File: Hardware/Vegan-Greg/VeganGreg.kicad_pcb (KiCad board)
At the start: 4 copper layers, 136 parts, among them J1 RBUS, J2 USB_C_Receptacle_USB2.0, J3 ServoCH0, J4 Conn_01x06_Socket, J5 GPIO Breakout, Q1 SSM3K15AMFV,L3F, U1 ESP32-S3, U2 SN65HVD230, U3 LM66200DRLR, U4 MAX77827AEFD+T, U5 SC4215ASTRT, U6 SIC438AED-T1, U7 LT1762, U8 TPS61089, Y1 R940000171

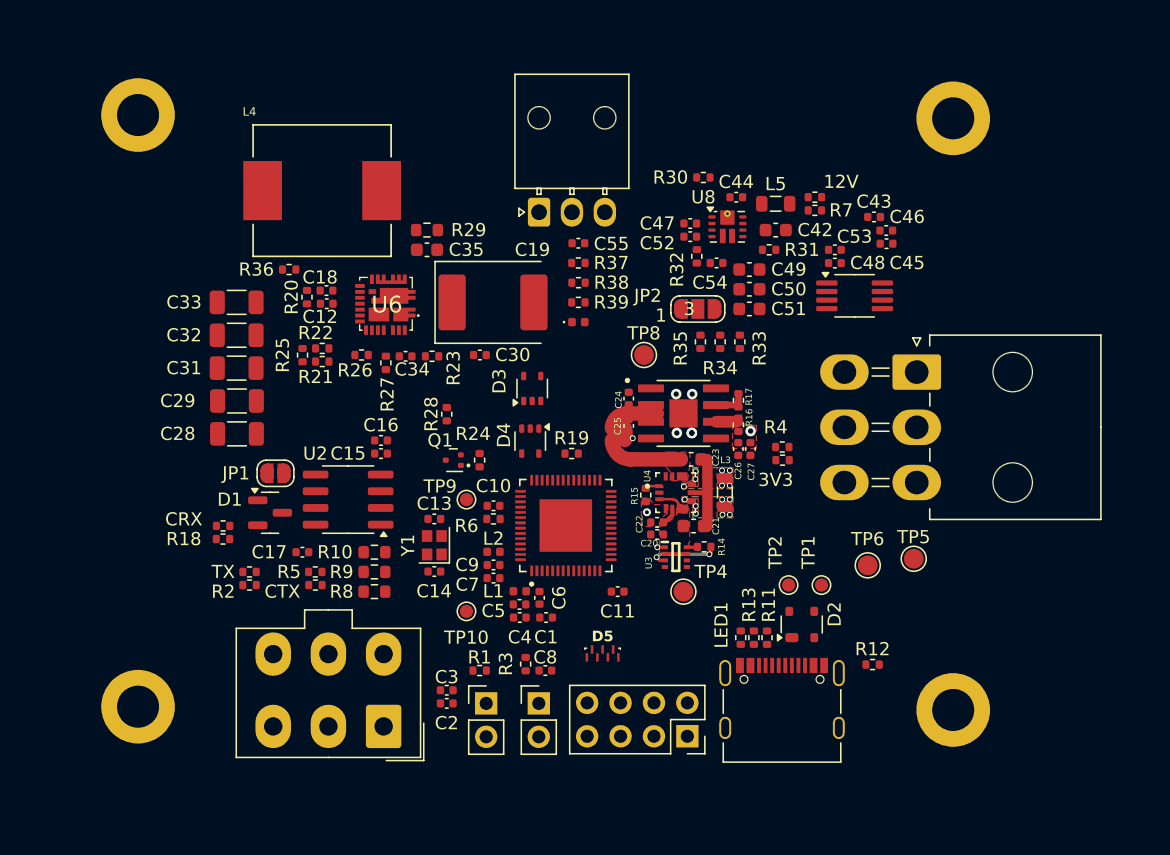
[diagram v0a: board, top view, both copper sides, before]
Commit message: Full PCB design
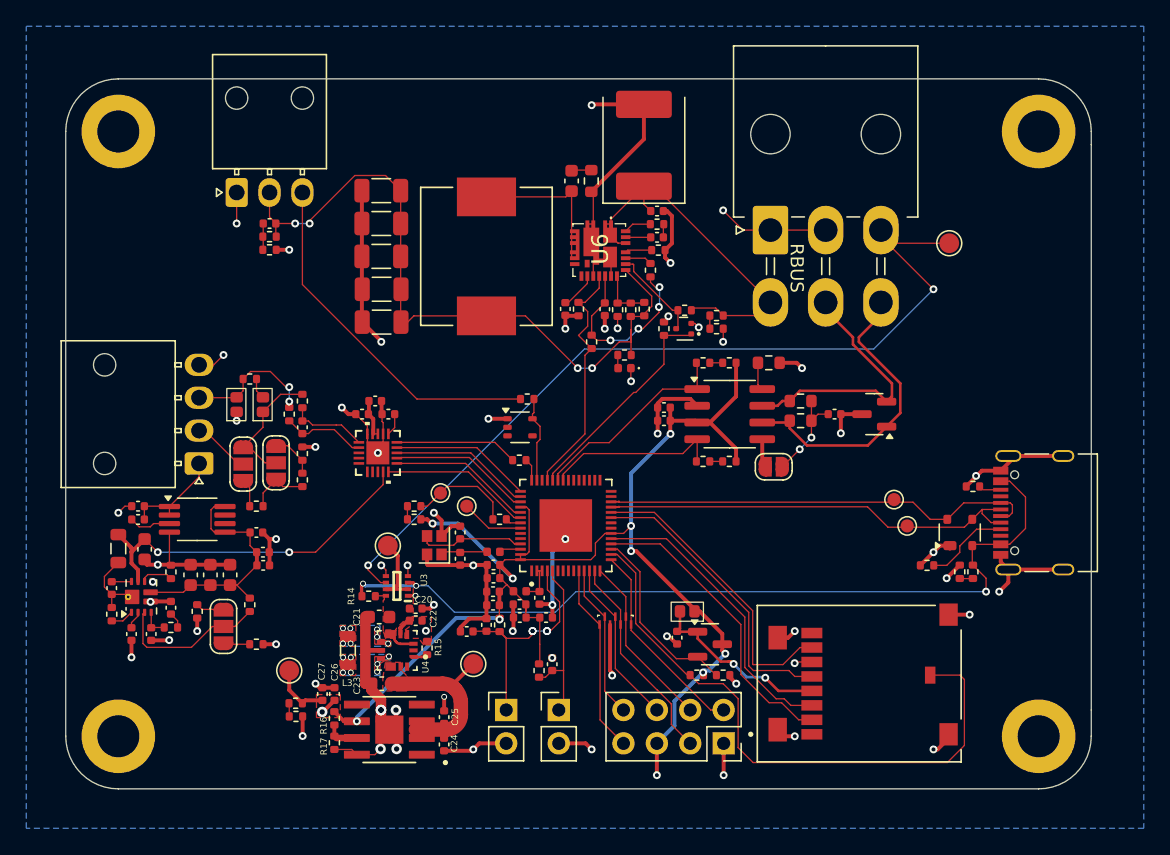
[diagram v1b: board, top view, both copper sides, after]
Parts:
- removed D3: ~, Package_TO_SOT_SMD:SOT-353_SC-70-5
- added C56: 10nF, Capacitor_SMD:C_0402_1005Metric, F.Cu at (134.9, 103.1)
- added C58: 220nF, Capacitor_SMD:C_0402_1005Metric, F.Cu at (141.5, 102.1)
- added C59: 1nF, Capacitor_SMD:C_0402_1005Metric, F.Cu at (140.5, 101.1)
- added C60: 1nF, Capacitor_SMD:C_0402_1005Metric, F.Cu at (139.5, 102.1)
- added C61: 0.1uF, Capacitor_SMD:C_0402_1005Metric, F.Cu at (163.4, 119.1)
- added J7: ST1W008S4TR2000, iclr:JAE_ST1W008S4TR2000, F.Cu at (177.4, 122.6)
- added JP13: SolderJumper_2_Open, iclr:SmallerSolderJP, F.Cu at (163.9, 117.1)
- added JP4: SolderJumper_3_Open, Jumper:SolderJumper-3_P1.3mm_Open_RoundedPad1.0x1.5mm_NumberLabels, F.Cu at (130.4, 105.9)
- added JP5: SolderJumper_3_Open, Jumper:SolderJumper-3_P1.3mm_Open_RoundedPad1.0x1.5mm_NumberLabels, F.Cu at (132.9, 105.8)
- added JP6: SolderJumper_2_Open, iclr:SmallerSolderJP, F.Cu at (131.9, 101.1)
- added JP7: SolderJumper_2_Open, iclr:SmallerSolderJP, F.Cu at (129.9, 101.1)
- added Q2: PMOS, Package_TO_SOT_SMD:SOT-23, F.Cu at (165.9, 119.6)
- added R46: 75k, Resistor_SMD:R_0402_1005Metric, F.Cu at (131.4, 109.1)
- added R47: 14k, Resistor_SMD:R_0402_1005Metric, F.Cu at (134.9, 107.1)
- added R48: 10k, Resistor_SMD:R_0402_1005Metric, F.Cu at (134.9, 105.1)
- added R49: 1k, Resistor_SMD:R_0402_1005Metric, F.Cu at (134.9, 101.1)
- added R50: 49.9, Resistor_SMD:R_0402_1005Metric, F.Cu at (130.9, 99.4)
- added R51: 1k, Resistor_SMD:R_0402_1005Metric, F.Cu at (133.9, 102.1)
- added R52: 54.9, Resistor_SMD:R_0402_1005Metric, F.Cu at (151.4, 105.6)
- added R59: 1k, Resistor_SMD:R_0402_1005Metric, F.Cu at (166.9, 121.9)
- added R60: 10k, Resistor_SMD:R_0402_1005Metric, F.Cu at (164.9, 121.9)
- added U9: ADS131M02IRUKR, footprints:WQFN20_ADS131_TEX, F.Cu at (140.7, 105.0)
- J1: footprint Connector_Molex:Molex_Mini-Fit_Jr_5566-06A_2x03_P4.20mm_Vertical -> iclr:Molex_Mini-Fit_Jr_5569-06A2_2x03_P4.20mm_Horizontal
- J4: value Conn_01x06_Socket -> 1053131104; footprint iclr:Molex_Mini-Fit_Jr_5569-06A2_2x03_P4.20mm_Horizontal -> Connector_Molex:Molex_Nano-Fit_105313-xx04_1x04_P2.50mm_Horizontal
- moved C48 56.5 mm to (122.4, 110.1)
- moved C53 56.5 mm to (122.4, 109.1)
- moved L5 56.5 mm to (120.9, 112.3), turned to -90 degrees
- moved C44 56.0 mm to (120.4, 115.3), turned to 90 degrees
- moved R30 55.9 mm to (120.4, 117.3), turned to -90 degrees
- moved J4 55.0 mm to (127.1, 105.8), turned to 180 degrees
- moved C42 53.8 mm to (122.9, 112.4), turned to -90 degrees
- moved C45 53.3 mm to (131.9, 113.6)
- moved C46 53.3 mm to (131.9, 112.6)
- moved U7 52.8 mm to (126.9, 110.1)
- moved C43 52.8 mm to (131.4, 111.1)
- moved C47 52.7 mm to (121.9, 118.8), turned to -90 degrees
- moved U8 52.7 mm to (122.7, 116.0), turned to 90 degrees
- moved R31 51.7 mm to (124.9, 114.1), turned to 90 degrees
- moved C52 50.9 mm to (123.4, 118.8), turned to -90 degrees
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- renumbered 12V to 12VLED1, 3V3 to 3V3LED1, CRX to CRXLED1, CTX to CTXLED1, TX to TXLED1, LED1 to USBLED1
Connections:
- C19 pad 1: +16.8V -> DeployV
- C30 pad 1: +16.8V -> DeployV
- C43 pad 1: Net-(U7-IN) -> 5_or_12
- C45 pad 1: /gregPart/LDO5.5V_IN -> 5_or_12
- C46 pad 1: /gregPart/LDO5.5V_IN -> 5_or_12
- C48 pad 1: Net-(U7-ADJ) -> LDO_out
- C49 pad 1: /gregPart/VOut - 5 or 12V -> 5_or_12
- C50 pad 1: /gregPart/VOut - 5 or 12V -> 5_or_12
- C51 pad 1: /gregPart/VOut - 5 or 12V -> 5_or_12
- C53 pad 1: Net-(U7-ADJ) -> LDO_out
- J1 pad 4: +25.2V -> DeployV
- J4 pad 1: GND -> LDO_out
- J4 pad 2: GND -> Net-(JP4-C)
- J4 pad 3: RBUS_uC_V -> Net-(JP7-B)
- J4 pad 4: +12V -> GND
- R28 pad 2: +16.8V -> DeployV
- R34 pad 1: /gregPart/VOut - 5 or 12V -> 5_or_12
- R7 pad 1: 25.2V -> DeployV
- U1 pad 16: unconnected-(U1-GPIO11/ADC2_CH0-Pad16) -> /SD_DET
- U1 pad 17: unconnected-(U1-GPIO12/ADC2_CH1-Pad17) -> /SD_EN
- U1 pad 18: unconnected-(U1-GPIO13/ADC2_CH2-Pad18) -> /SD_CS
- U1 pad 19: unconnected-(U1-GPIO14/ADC2_CH3-Pad19) -> /VSPI_MOSI
- U1 pad 23: unconnected-(U1-GPIO17/ADC2_CH6/DAC_2-Pad23) -> /VSPI_SCLK
- U1 pad 24: unconnected-(U1-GPIO18/ADC2_CH7/DAC_1-Pad24) -> /VSPI_MISO
- U1 pad 36: unconnected-(U1-SPICLK_N/GPIO48-Pad36) -> /CAN_RX
- U1 pad 37: /BuckPGOOD -> /CAN_TX
- U1 pad 38: /CAN_TX -> /BUCK_EN
- U1 pad 39: /CAN_RX -> /BuckPGOOD
- U1 pad 42: unconnected-(U1-GPIO37-Pad42) -> Net-(U1-GPIO37)
- U1 pad 43: /BUCK_EN -> /ADS_MOSI
- U1 pad 44: unconnected-(U1-MTCK/JTAG/GPIO39-Pad44) -> /ADS_MISO
- U1 pad 45: unconnected-(U1-MTDO/JTAG/GPIO40-Pad45) -> /ADS_SCLK
- U1 pad 47: unconnected-(U1-MTDI/JTAG/GPIO41-Pad47) -> /ADS_DRDY
- U1 pad 48: unconnected-(U1-MTMS/JTAG/GPIO42-Pad48) -> /ADS_CS
- U6 pad 1: +16.8V -> DeployV
- U6 pad 2: +16.8V -> DeployV
- U6 pad 22: +16.8V -> DeployV
- U6 pad 26: +16.8V -> DeployV
- U7 pad 1: Net-(U7-ADJ) -> LDO_out
- U7 pad 2: Net-(U7-ADJ) -> LDO_out
- U7 pad 5: Net-(U7-IN) -> 5_or_12
- U7 pad 8: Net-(U7-IN) -> 5_or_12
- U8 pad 6: /gregPart/VOut - 5 or 12V -> 5_or_12
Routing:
- net GND: track 7.31 -> 202.4 mm, vias 8 -> 64
- net +3V3: track 1.61 -> 110.5 mm, vias 1 -> 11
- net RBUS_uC_V: track 0.00 -> 65.1 mm, vias 0 -> 2
- net VBUS: track 5.51 -> 63.7 mm, vias 2 -> 3
- net +6V: track 0.00 -> 54.8 mm, vias 0 -> 4
- net /SD_DET: track 0.00 -> 46.1 mm
- net /Data+: track 0.00 -> 33.9 mm
- net /Data-: track 0.00 -> 33.5 mm
- net DeployV: track 0.00 -> 31.8 mm
- net +3.3V: track 0.00 -> 30.5 mm, vias 0 -> 3
- net Net-(J3-Pin_3): track 0.00 -> 27.2 mm
- net /VSPI_MOSI: track 0.00 -> 23.3 mm
- net /SD_CS: track 0.00 -> 23.0 mm
- net /VSPI_MISO: track 0.00 -> 23.0 mm
- net /VSPI_SCLK: track 0.00 -> 22.7 mm
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- added copper zone on In2.Cu, net +3.3V
- added copper zone on B.Cu, net GND
- added copper zone on In1.Cu, net GND
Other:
- board outline added: 78 x 54 mm
